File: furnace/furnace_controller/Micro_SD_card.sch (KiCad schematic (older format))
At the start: 7 parts, among them J12 PLS-5, J13 CTF-11081-P

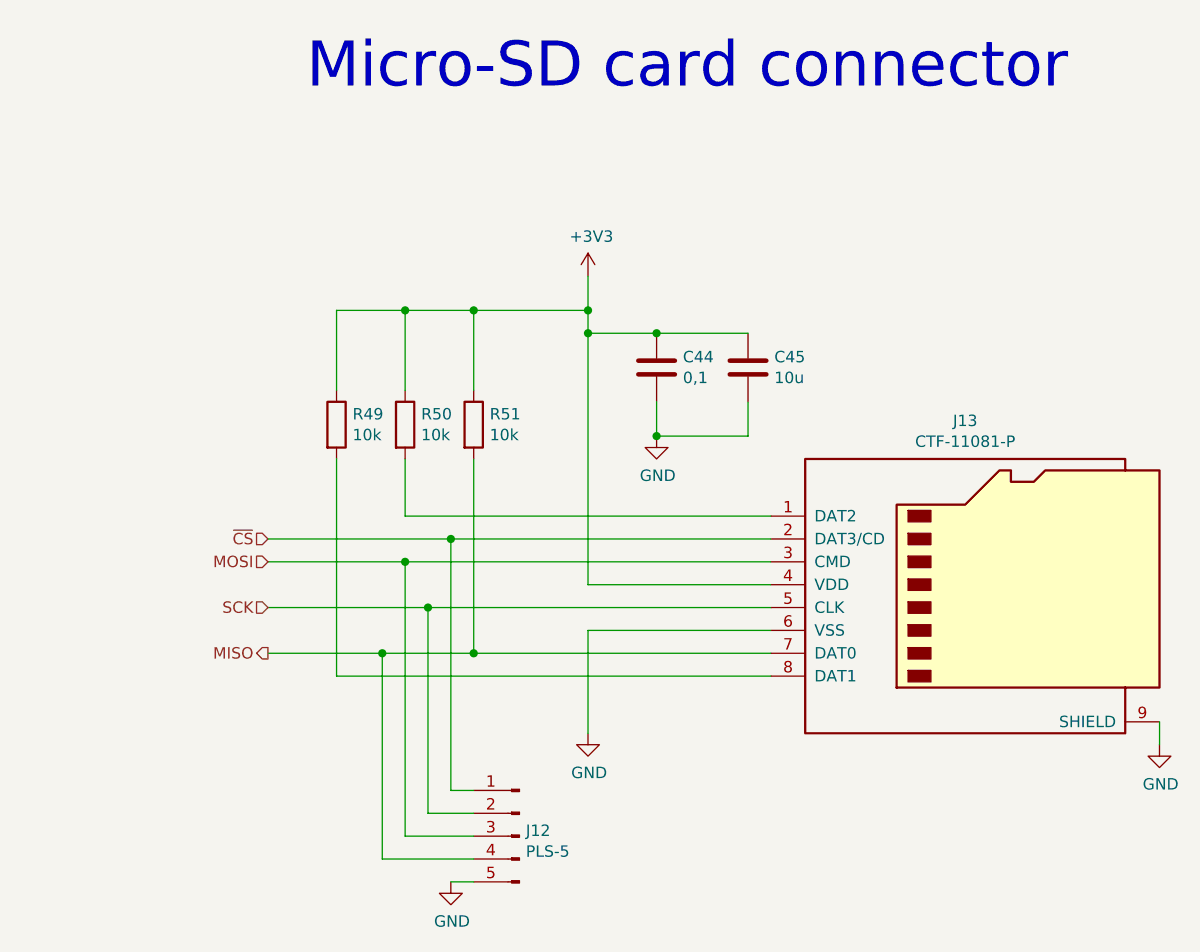
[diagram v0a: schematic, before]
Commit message: Add files via upload
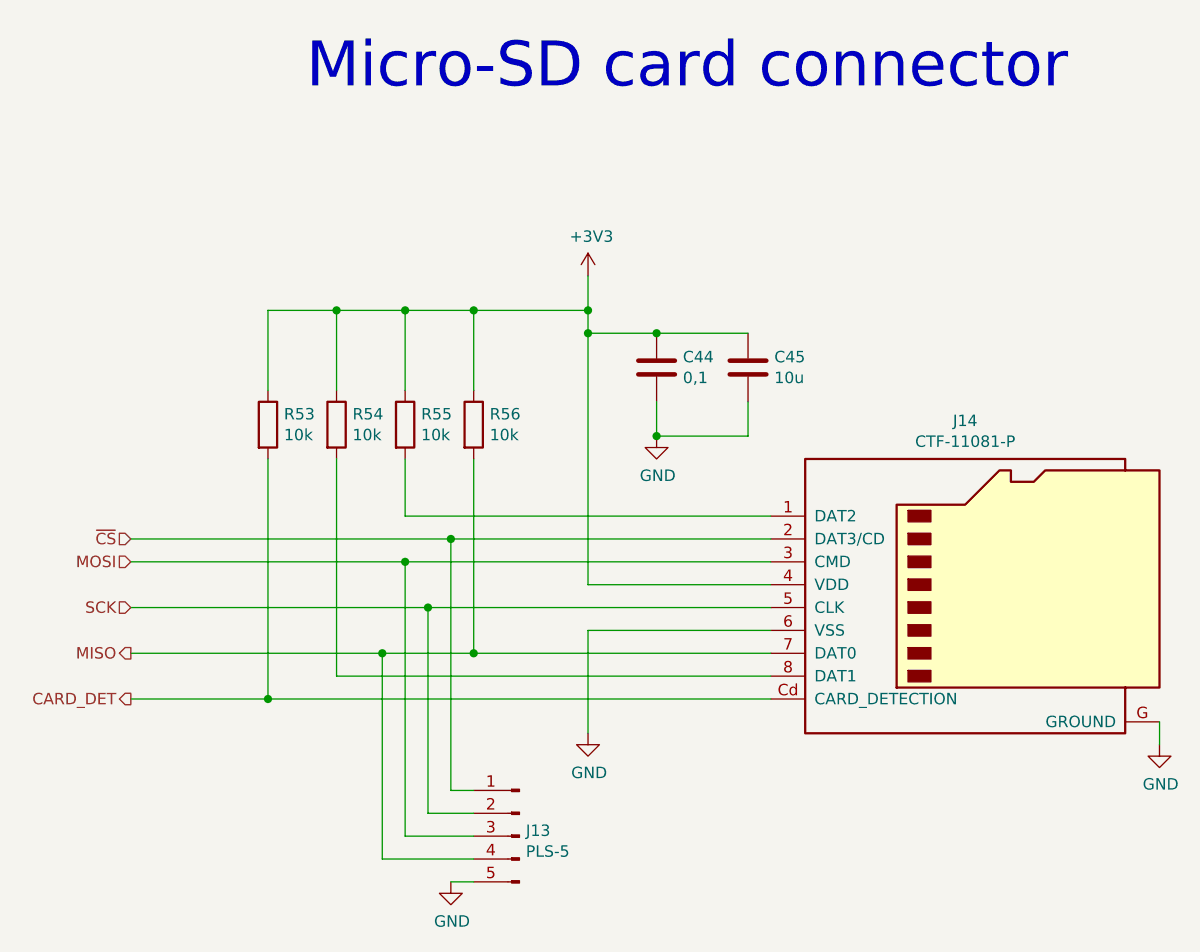
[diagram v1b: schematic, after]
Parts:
- removed J13: CTF-11081-P, symbol Connector:Micro_SD_Card
- added J14: CTF-11081-P, furnace_controller:CTF-11081-P, symbol Micro_SD_card:CTF-11081-P
- added R53: 10k, Resistor_SMD:R_0603_1608Metric_Pad0.98x0.95mm_HandSolder, symbol Device:R
- C44: footprint Capacitor_SMD:C_0603_1608Metric_Pad1.05x0.95mm_HandSolder -> Capacitor_SMD:C_0603_1608Metric_Pad1.08x0.95mm_HandSolder
- C45: footprint Capacitor_SMD:C_1206_3216Metric_Pad1.42x1.75mm_HandSolder -> Capacitor_SMD:C_1206_3216Metric_Pad1.33x1.80mm_HandSolder
- R54: renamed from R49; footprint Resistor_SMD:R_0603_1608Metric_Pad1.05x0.95mm_HandSolder -> Resistor_SMD:R_0603_1608Metric_Pad0.98x0.95mm_HandSolder
- R55: renamed from R50; footprint Resistor_SMD:R_0603_1608Metric_Pad1.05x0.95mm_HandSolder -> Resistor_SMD:R_0603_1608Metric_Pad0.98x0.95mm_HandSolder
- R56: renamed from R51; footprint Resistor_SMD:R_0603_1608Metric_Pad1.05x0.95mm_HandSolder -> Resistor_SMD:R_0603_1608Metric_Pad0.98x0.95mm_HandSolder
- renumbered J12 to J13
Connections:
- net +3V3: now also J14.4 (VDD), R53.1
- net GND: now also J14.6 (VSS), J14.G (GROUND)
- net MISO: now also J14.7 (DAT0)
- net MOSI: now also J14.3 (CMD)
- net SCK: now also J14.5 (CLK)
- net ~CS~: now also J14.2 (DAT3/CD)
- net at R55.2: now also J14.1 (DAT2)
- net at R54.2: now also J14.8 (DAT1)
- new net CARD_DET: J14.Cd (CARD_DETECTION), R53.2
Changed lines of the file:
@@
 $Descr A4 11693 8268
 encoding utf-8
-Sheet 15 18
+Sheet 18 18
 Title "Furnace controller"
-Date "2021-08-26"
+Date "2021-09-24"
 Rev "1.0"
 Comp "Yuriy Volkov"
@@
 $EndDescr
 $Comp
-L Connector:Micro_SD_Card J?
-U 1 1 60B1D1CB
-P 7200 4600
-AR Path="/60B1D1CB" Ref="J?"  Part="1"
-AR Path="/609C9D41/60B1D1CB" Ref="J?"  Part="1"
-AR Path="/60B1951B/60B1D1CB" Ref="J13"  Part="1"
-F 0 "J13" H 7150 5317 50  0000 C CNN
-F 1 "CTF-11081-P" H 7150 5226 50  0000 C CNN
-F 2 "" H 8350 4900 50  0001 C CNN
-F 3 "http://katalog.we-online.de/em/datasheet/693072010801.pdf" H 7200 4600 50  0001 C CNN
-	1    7200 4600
-	1    0    0    -1
-$EndComp
-$Comp
 L Device:R R?
 U 1 1 60B1D1D1
@@
 AR Path="/60B1D1D1" Ref="R?"  Part="1"
 AR Path="/609C9D41/60B1D1D1" Ref="R?"  Part="1"
-AR Path="/60B1951B/60B1D1D1" Ref="R51"  Part="1"
-F 0 "R51" H 5070 3946 50  0000 L CNN
+AR Path="/60B1951B/60B1D1D1" Ref="R56"  Part="1"
+F 0 "R56" H 5070 3946 50  0000 L CNN
 F 1 "10k" H 5070 3855 50  0000 L CNN
-F 2 "Resistor_SMD:R_0603_1608Metric_Pad1.05x0.95mm_HandSolder" V 4930 3900 50  0001 C CNN
+F 2 "Resistor_SMD:R_0603_1608Metric_Pad0.98x0.95mm_HandSolder" V 4930 3900 50  0001 C CNN
 F 3 "~" H 5000 3900 50  0001 C CNN
 	1    5000 3900
@@
 AR Path="/60B1D1D7" Ref="#PWR?"  Part="1"
 AR Path="/609C9D41/60B1D1D7" Ref="#PWR?"  Part="1"
-AR Path="/60B1951B/60B1D1D7" Ref="#PWR056"  Part="1"
-F 0 "#PWR056" H 8000 5050 50  0001 C CNN
+AR Path="/60B1951B/60B1D1D7" Ref="#PWR061"  Part="1"
+F 0 "#PWR061" H 8000 5050 50  0001 C CNN
 F 1 "GND" H 8005 5127 50  0000 C CNN
 F 2 "" H 8000 5300 50  0001 C CNN
@@
 F 0 "C44" H 5915 3696 50  0000 L CNN
 F 1 "0,1" H 5915 3605 50  0000 L CNN
-F 2 "Capacitor_SMD:C_0603_1608Metric_Pad1.05x0.95mm_HandSolder" H 5838 3500 50  0001 C CNN
+F 2 "Capacitor_SMD:C_0603_1608Metric_Pad1.08x0.95mm_HandSolder" H 5838 3500 50  0001 C CNN
 F 3 "~" H 5800 3650 50  0001 C CNN
 	1    5800 3650
@@
 AR Path="/60B1D1E3" Ref="#PWR?"  Part="1"
 AR Path="/609C9D41/60B1D1E3" Ref="#PWR?"  Part="1"
-AR Path="/60B1951B/60B1D1E3" Ref="#PWR054"  Part="1"
-F 0 "#PWR054" H 5500 5000 50  0001 C CNN
+AR Path="/60B1951B/60B1D1E3" Ref="#PWR059"  Part="1"
+F 0 "#PWR059" H 5500 5000 50  0001 C CNN
 F 1 "GND" H 5505 5077 50  0000 C CNN
 F 2 "" H 5500 5250 50  0001 C CNN
@@
 AR Path="/609FED99/60B1D1E9" Ref="#PWR?"  Part="1"
 AR Path="/609C9D41/60B1D1E9" Ref="#PWR?"  Part="1"
-AR Path="/60B1951B/60B1D1E9" Ref="#PWR053"  Part="1"
-F 0 "#PWR053" H 5500 3100 50  0001 C CNN
+AR Path="/60B1951B/60B1D1E9" Ref="#PWR058"  Part="1"
+F 0 "#PWR058" H 5500 3100 50  0001 C CNN
 F 1 "+3V3" H 5515 3423 50  0000 C CNN
 F 2 "" H 5500 3250 50  0001 C CNN
@@
 AR Path="/60B1D1EF" Ref="#PWR?"  Part="1"
 AR Path="/609C9D41/60B1D1EF" Ref="#PWR?"  Part="1"
-AR Path="/60B1951B/60B1D1EF" Ref="#PWR055"  Part="1"
-F 0 "#PWR055" H 5800 3700 50  0001 C CNN
+AR Path="/60B1951B/60B1D1EF" Ref="#PWR060"  Part="1"
+F 0 "#PWR060" H 5800 3700 50  0001 C CNN
 F 1 "GND" H 5805 3777 50  0000 C CNN
 F 2 "" H 5800 3950 50  0001 C CNN
@@
 AR Path="/60B1D208" Ref="R?"  Part="1"
 AR Path="/609C9D41/60B1D208" Ref="R?"  Part="1"
-AR Path="/60B1951B/60B1D208" Ref="R50"  Part="1"
-F 0 "R50" H 4770 3946 50  0000 L CNN
+AR Path="/60B1951B/60B1D208" Ref="R55"  Part="1"
+F 0 "R55" H 4770 3946 50  0000 L CNN
 F 1 "10k" H 4770 3855 50  0000 L CNN
-F 2 "Resistor_SMD:R_0603_1608Metric_Pad1.05x0.95mm_HandSolder" V 4630 3900 50  0001 C CNN
+F 2 "Resistor_SMD:R_0603_1608Metric_Pad0.98x0.95mm_HandSolder" V 4630 3900 50  0001 C CNN
 F 3 "~" H 4700 3900 50  0001 C CNN
 	1    4700 3900
@@
 AR Path="/60B1D20E" Ref="R?"  Part="1"
 AR Path="/609C9D41/60B1D20E" Ref="R?"  Part="1"
-AR Path="/60B1951B/60B1D20E" Ref="R49"  Part="1"
-F 0 "R49" H 4470 3946 50  0000 L CNN
+AR Path="/60B1951B/60B1D20E" Ref="R54"  Part="1"
+F 0 "R54" H 4470 3946 50  0000 L CNN
 F 1 "10k" H 4470 3855 50  0000 L CNN
-F 2 "Resistor_SMD:R_0603_1608Metric_Pad1.05x0.95mm_HandSolder" V 4330 3900 50  0001 C CNN
+F 2 "Resistor_SMD:R_0603_1608Metric_Pad0.98x0.95mm_HandSolder" V 4330 3900 50  0001 C CNN
 F 3 "~" H 4400 3900 50  0001 C CNN
 	1    4400 3900
@@
 F 0 "C45" H 6315 3696 50  0000 L CNN
 F 1 "10u" H 6315 3605 50  0000 L CNN
-F 2 "Capacitor_SMD:C_1206_3216Metric_Pad1.42x1.75mm_HandSolder" H 6238 3500 50  0001 C CNN
+F 2 "Capacitor_SMD:C_1206_3216Metric_Pad1.33x1.80mm_HandSolder" H 6238 3500 50  0001 C CNN
 F 3 "~" H 6200 3650 50  0001 C CNN
 	1    6200 3650
@@
 Connection ~ 5800 3950
 Wire Wire Line
-	4100 4400 4900 4400
-Wire Wire Line
-	4100 4500 4700 4500
-Wire Wire Line
-	4100 4700 4800 4700
-Wire Wire Line
-	4100 4900 4600 4900
+	3500 4400 4900 4400
+Wire Wire Line
+	3500 4500 4700 4500
+Wire Wire Line
+	3500 4700 4800 4700
+Wire Wire Line
+	3500 4900 4600 4900
 Connection ~ 5000 4900
 Text Notes 7600 2450 2    197  ~ 0
 Micro-SD card connector
-Text HLabel 4100 4400 0    50   Input ~ 0
+Text HLabel 3500 4400 0    50   Input ~ 0
 ~CS~
-Text HLabel 4100 4500 0    50   Input ~ 0
+Text HLabel 3500 4500 0    50   Input ~ 0
 MOSI
-Text HLabel 4100 4700 0    50   Input ~ 0
+Text HLabel 3500 4700 0    50   Input ~ 0
 SCK
-Text HLabel 4100 4900 0    50   Output ~ 0
+Text HLabel 3500 4900 0    50   Output ~ 0
 MISO
 $Comp
-L Connector:Conn_01x05_Male J12
+L Connector:Conn_01x05_Male J13
 U 1 1 60B35003
 P 5200 5700
-F 0 "J12" H 5172 5724 50  0000 R CNN
+F 0 "J13" H 5172 5724 50  0000 R CNN
 F 1 "PLS-5" H 5172 5633 50  0000 R CNN
 F 2 "Connector_PinHeader_2.54mm:PinHeader_1x05_P2.54mm_Vertical" H 5200 5700 50  0001 C CNN
@@
 AR Path="/60B38C7E" Ref="#PWR?"  Part="1"
 AR Path="/609C9D41/60B38C7E" Ref="#PWR?"  Part="1"
-AR Path="/60B1951B/60B38C7E" Ref="#PWR052"  Part="1"
-F 0 "#PWR052" H 4900 5650 50  0001 C CNN
+AR Path="/60B1951B/60B38C7E" Ref="#PWR057"  Part="1"
+F 0 "#PWR057" H 4900 5650 50  0001 C CNN
 F 1 "GND" H 4905 5727 50  0000 C CNN
 F 2 "" H 4900 5900 50  0001 C CNN
@@
 	1    0    0    -1
 $EndComp
+$Comp
+L Micro_SD_card:CTF-11081-P J14
+U 1 1 613E2B59
+P 7200 4600
+F 0 "J14" H 7150 5317 50  0000 C CNN
+F 1 "CTF-11081-P" H 7150 5226 50  0000 C CNN
+F 2 "furnace_controller:CTF-11081-P" H 8350 4900 50  0001 C CNN
+F 3 "" H 7200 4600 50  0001 C CNN
+	1    7200 4600
+	1    0    0    -1
+$EndComp
+Text HLabel 3500 5100 0    50   Output ~ 0
+CARD_DET
+$Comp
+L Device:R R?
+U 1 1 613EBA2B
+P 4100 3900
+AR Path="/613EBA2B" Ref="R?"  Part="1"
+AR Path="/609C9D41/613EBA2B" Ref="R?"  Part="1"
+AR Path="/60B1951B/613EBA2B" Ref="R53"  Part="1"
+F 0 "R53" H 4170 3946 50  0000 L CNN
+F 1 "10k" H 4170 3855 50  0000 L CNN
+F 2 "Resistor_SMD:R_0603_1608Metric_Pad0.98x0.95mm_HandSolder" V 4030 3900 50  0001 C CNN
+F 3 "~" H 4100 3900 50  0001 C CNN
+	1    4100 3900
+	1    0    0    -1
+$EndComp
+Wire Wire Line
+	4400 3400 4100 3400
+Wire Wire Line
+	4100 3400 4100 3750
+Connection ~ 4400 3400
+Wire Wire Line
+	6300 5100 4100 5100
+Wire Wire Line
+	4100 4050 4100 5100
+Connection ~ 4100 5100
+Wire Wire Line
+	4100 5100 3500 5100
 $EndSCHEMATC
